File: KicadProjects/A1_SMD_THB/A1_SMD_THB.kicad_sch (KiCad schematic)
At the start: 1 part

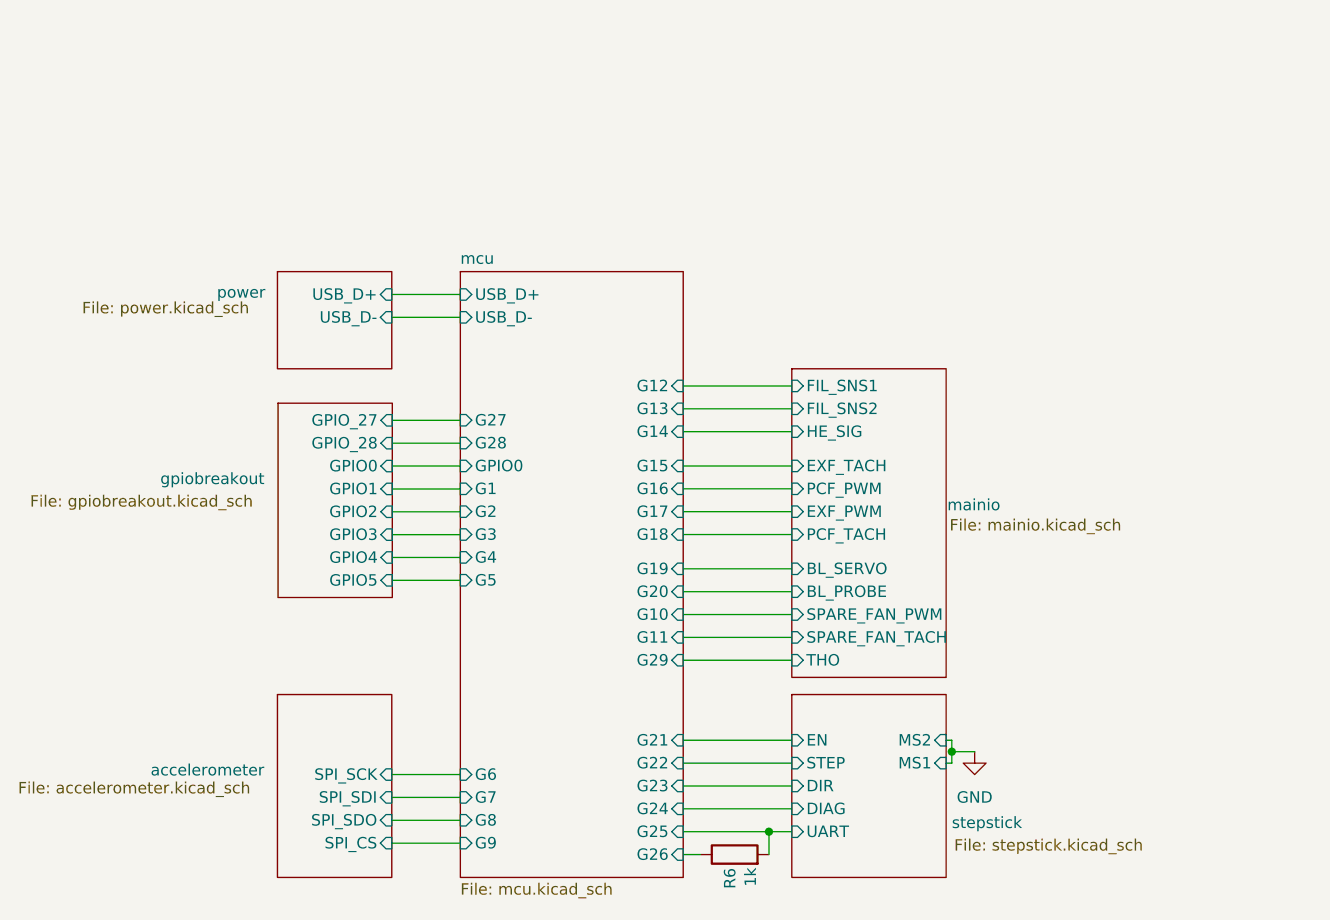
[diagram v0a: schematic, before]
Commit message: e
e
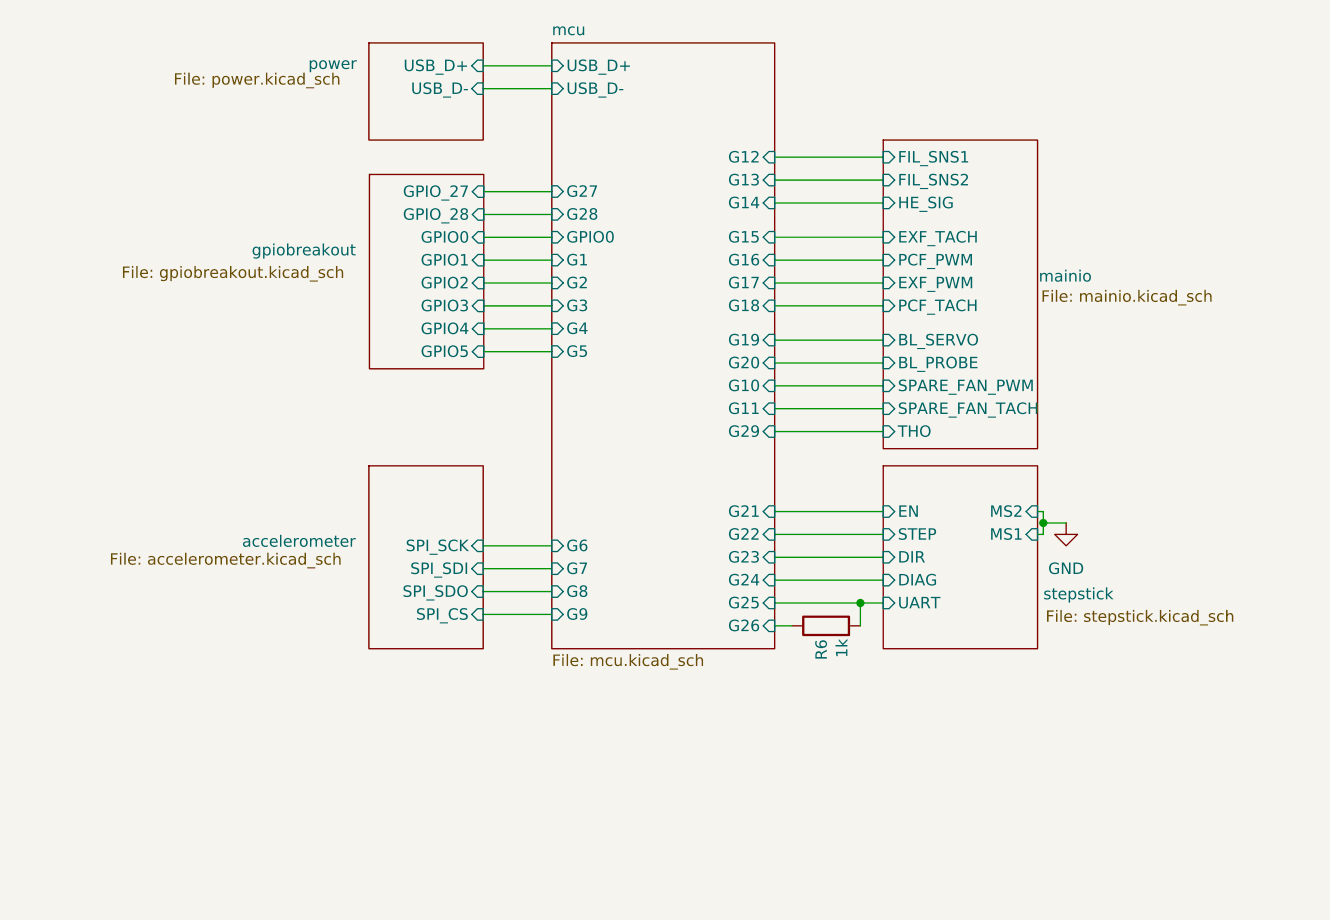
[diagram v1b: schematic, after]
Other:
- moved on the sheet: R6
